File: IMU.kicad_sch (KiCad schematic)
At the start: 0 parts

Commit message: Protocolos I2C/SPI
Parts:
- added U3: 4754, 4754:MODULE_4754, symbol 4754:4754
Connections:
- new net +5V: U3.JP1_1 (VIN), U3.JP2_2 (P0), U3.JP2_3 (P1)
- new net GND: U3.JP1_3 (GND)
- new net IMU INT: U3.JP1_6 (~{INT})
- new net IMU RST: U3.JP2_4 (~{RST})
- new net SPI1_CSK: U3.JP1_4 (SCL)
- new net SPI1_MISO: U3.JP2_5 (DI)
- new net SPI1_MOSI: U3.JP1_5 (SDA)
- new net SPI1_NSS: U3.JP2_6 (CS)
- no-connect marks 0 -> 2

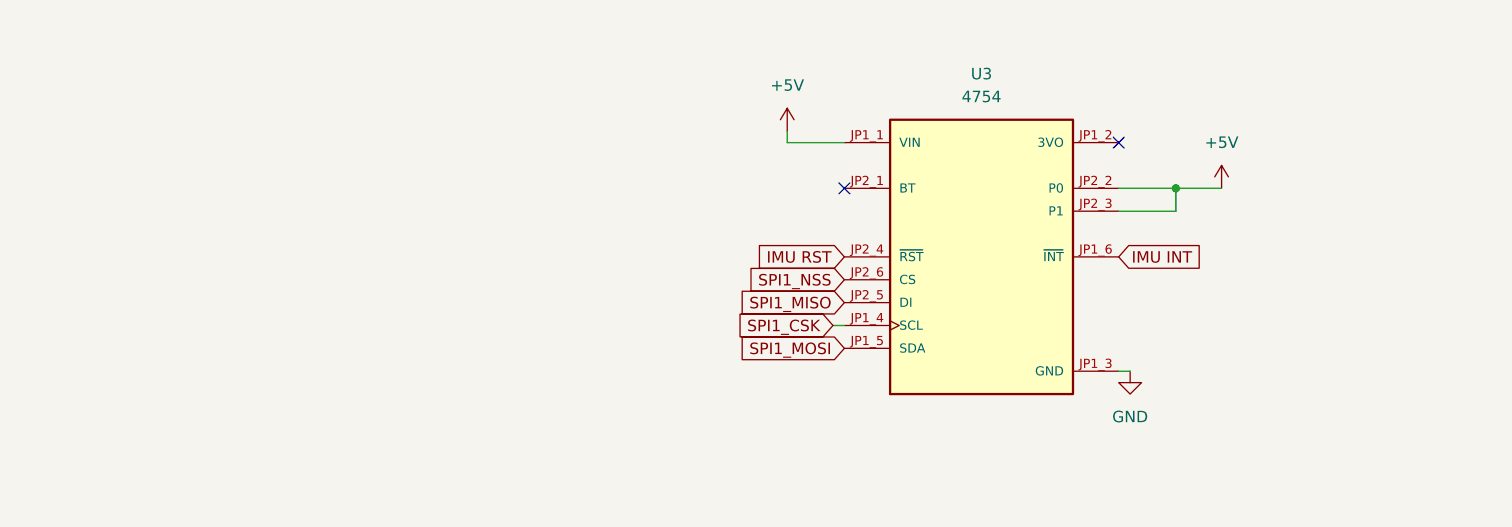
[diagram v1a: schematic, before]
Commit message: BECERRA
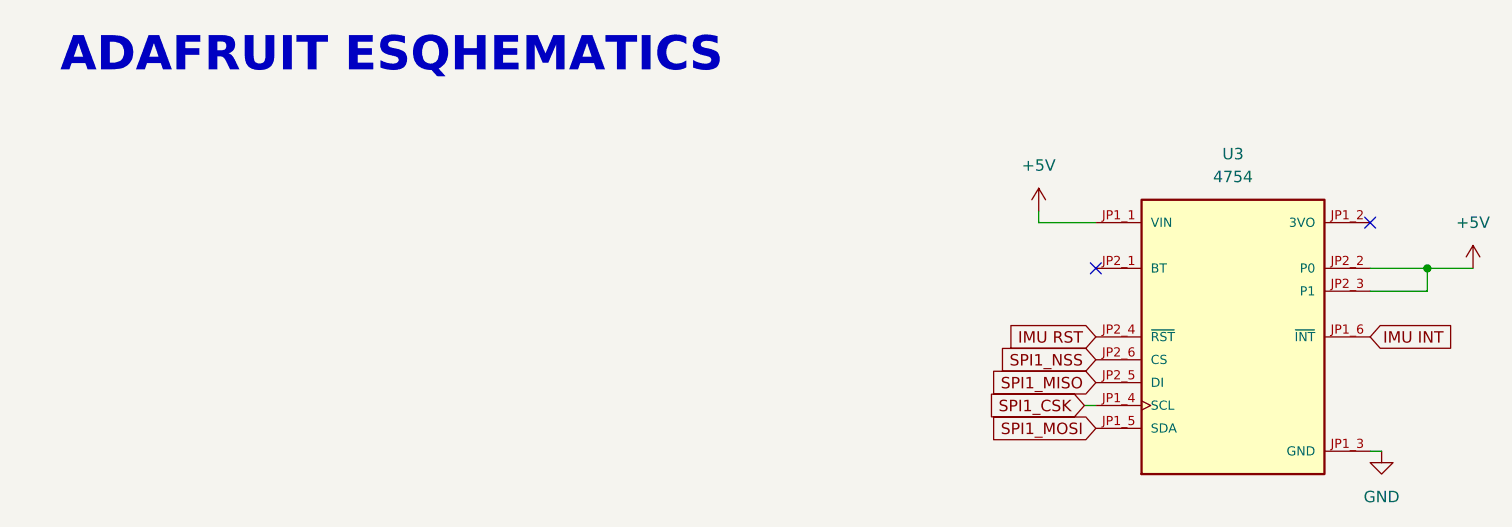
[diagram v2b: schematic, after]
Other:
- note added: "ADAFRUIT ESQHEMATICS"
- moved on the sheet: U3
